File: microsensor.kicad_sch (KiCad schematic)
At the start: 23 parts, among them J1 ARM SWD, Q1 IRLML2244TRPBF, SW1 Control, U1 HDC2080, U3 NORA B206, Y1 32768

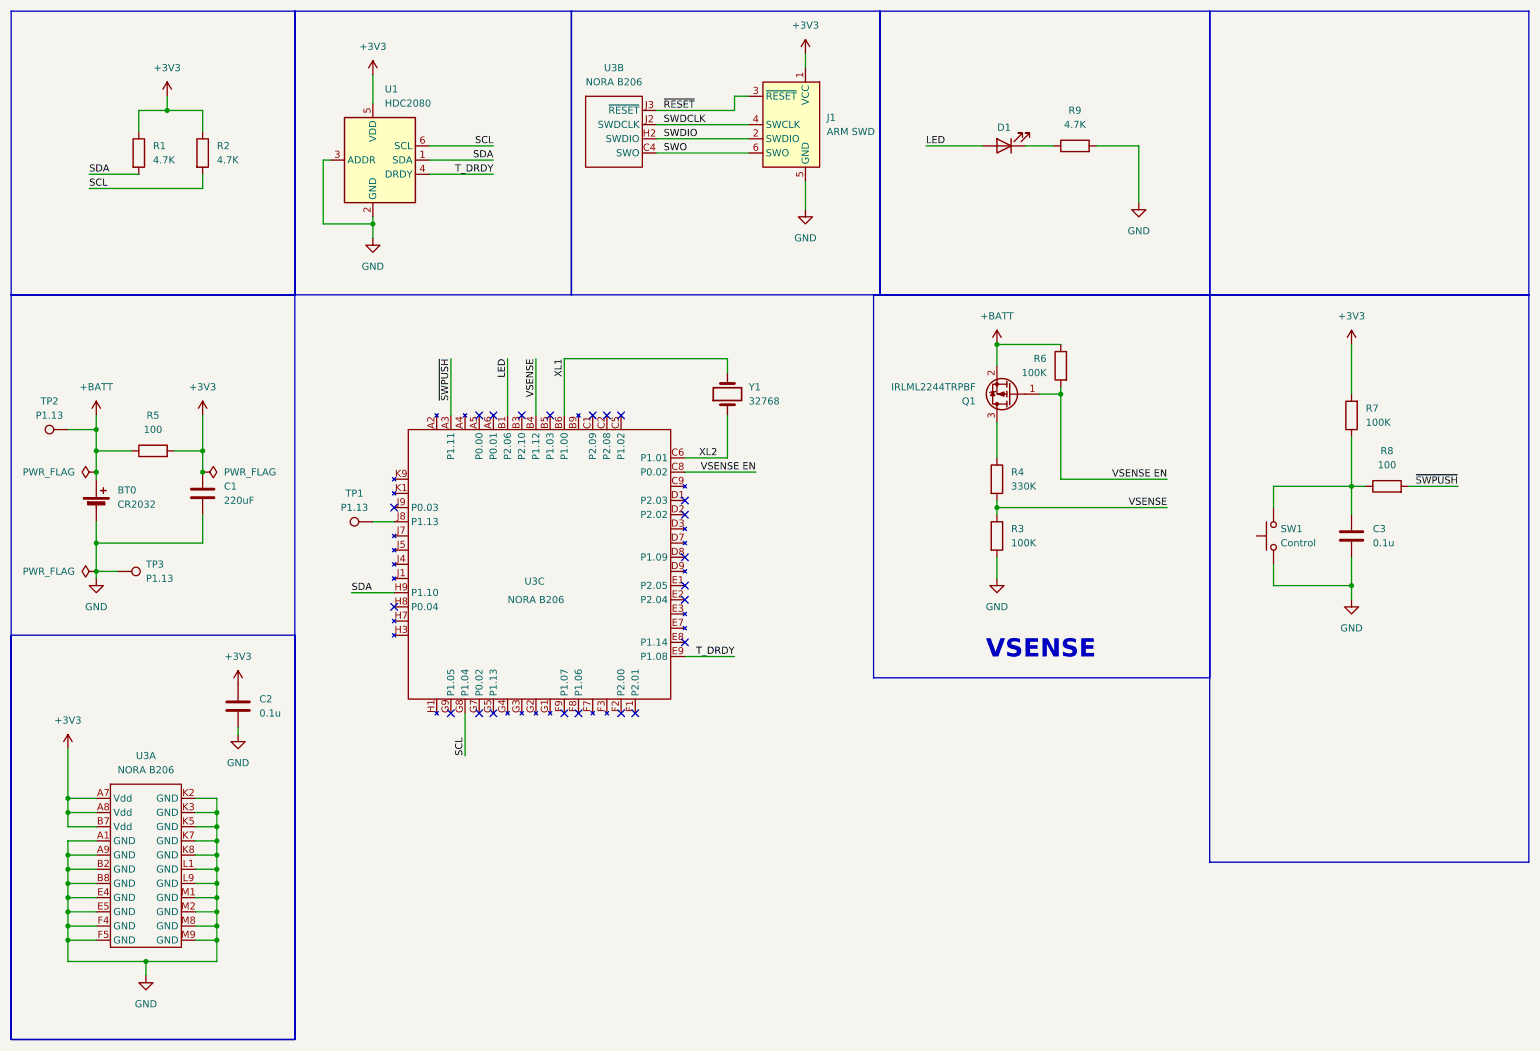
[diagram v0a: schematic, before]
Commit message: Put TP together, minor refactors, added more dimensions
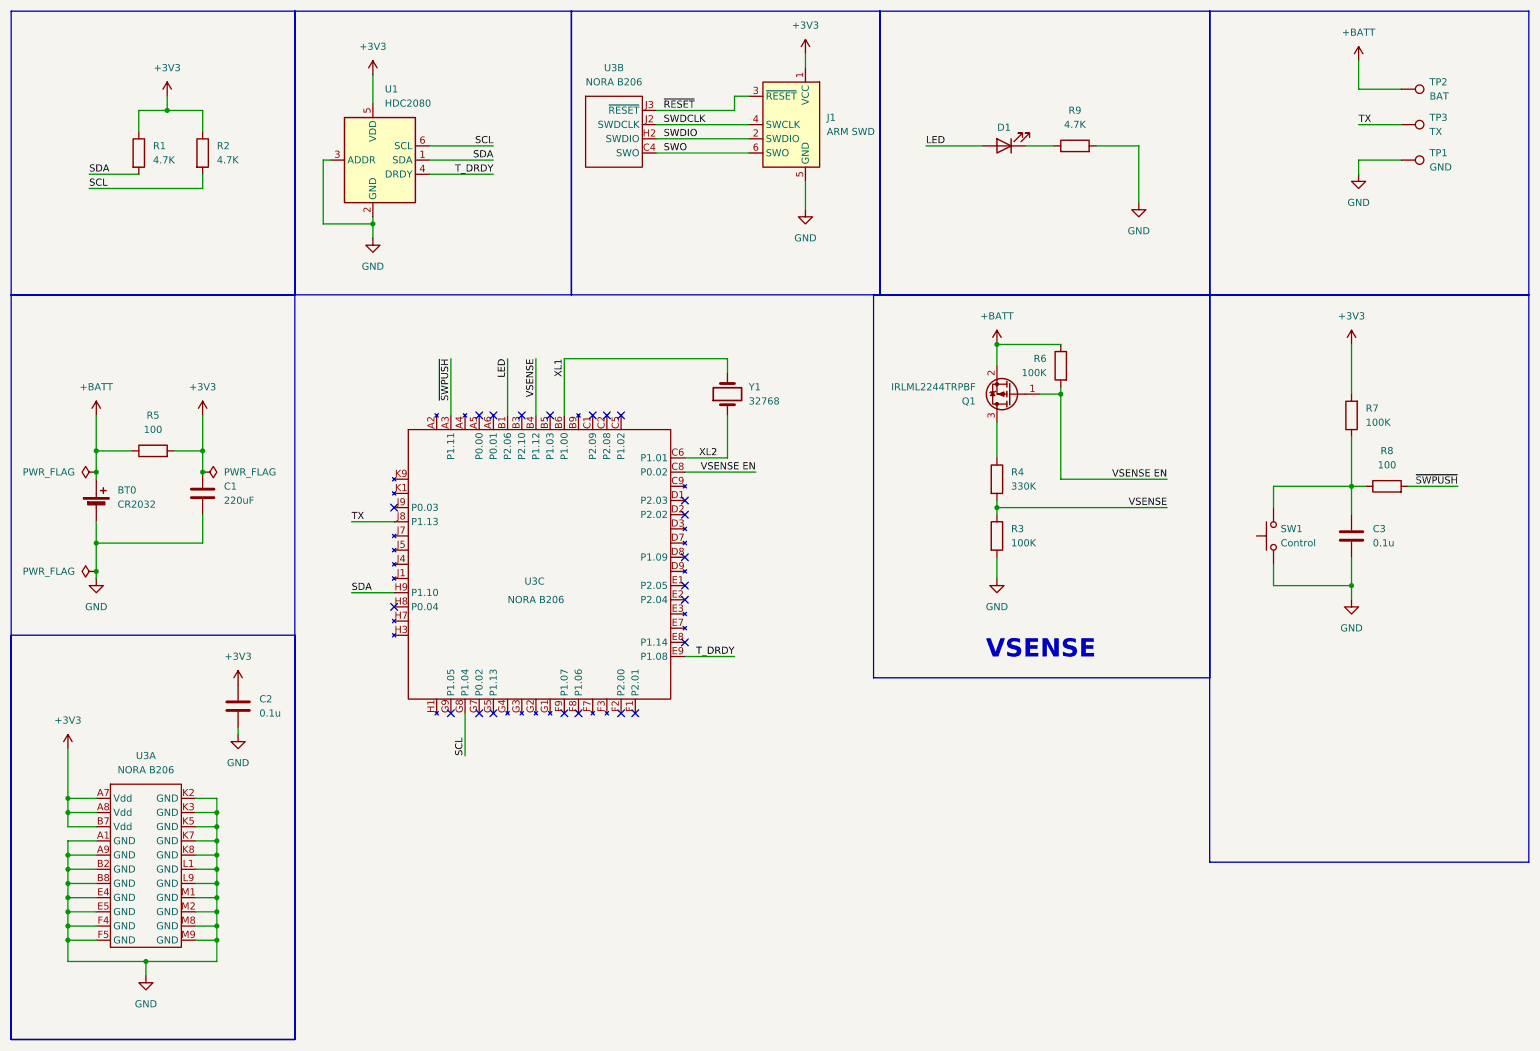
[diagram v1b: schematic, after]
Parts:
- TP1: renamed from TP3; value P1.13 -> GND
- TP2: value P1.13 -> BAT
- TP3: renamed from TP1; value P1.13 -> TX
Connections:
- net TX: now reaches TP3.1, U3.J8 (P1.13)
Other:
- moved on the sheet: TP1, TP2, TP3
